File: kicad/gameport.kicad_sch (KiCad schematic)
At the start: 0 parts

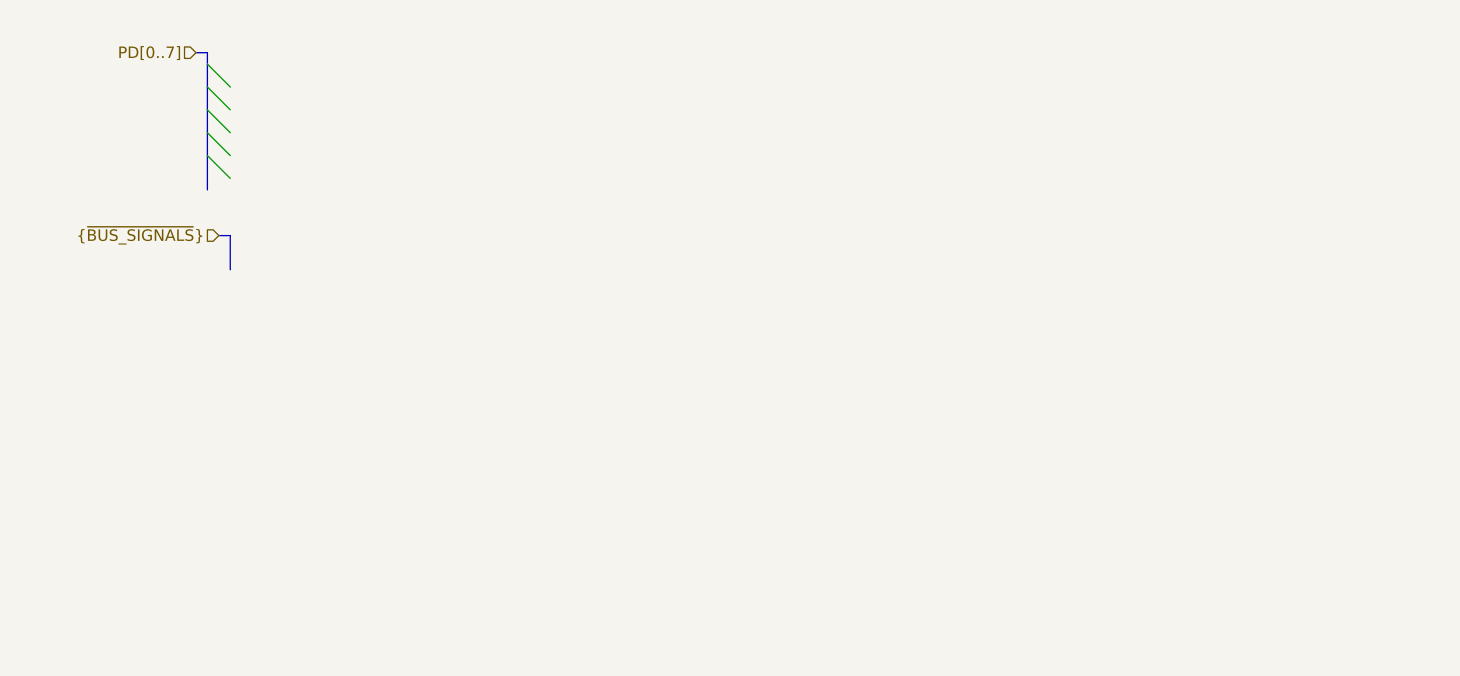
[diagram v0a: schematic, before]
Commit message: update kicad project
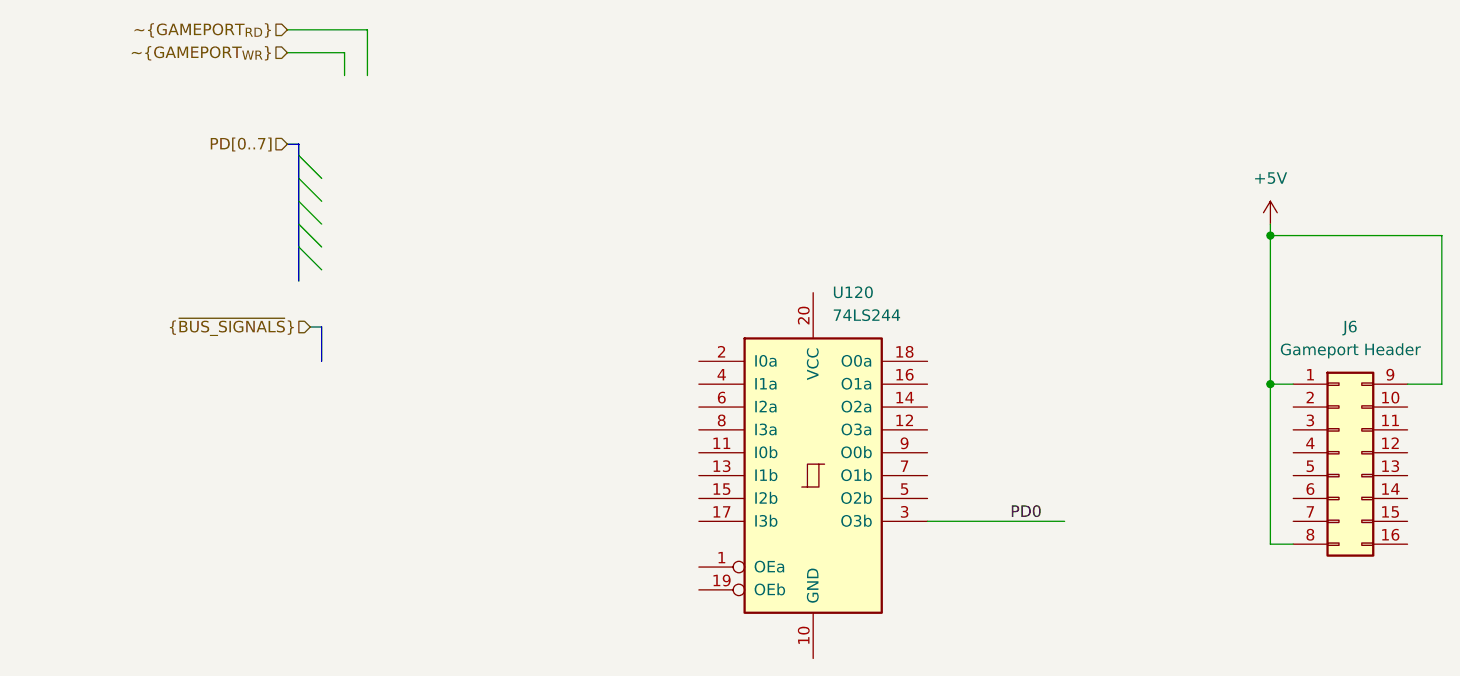
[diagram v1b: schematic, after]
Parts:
- added J6: Gameport Header, seequa_footprints:PinHeader_Gameport_Vertical, symbol seequa:Gameport Header
- added U120: 74LS244, Package_DIP:DIP-20_W7.62mm_Socket, symbol 74xx:74LS244
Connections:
- new net +5V: J6.1 (+5V), J6.8 (+5V), J6.9 (+5V)
- new net PD0: U120.3 (O3b)
